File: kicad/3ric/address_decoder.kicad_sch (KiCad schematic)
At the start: 29 parts

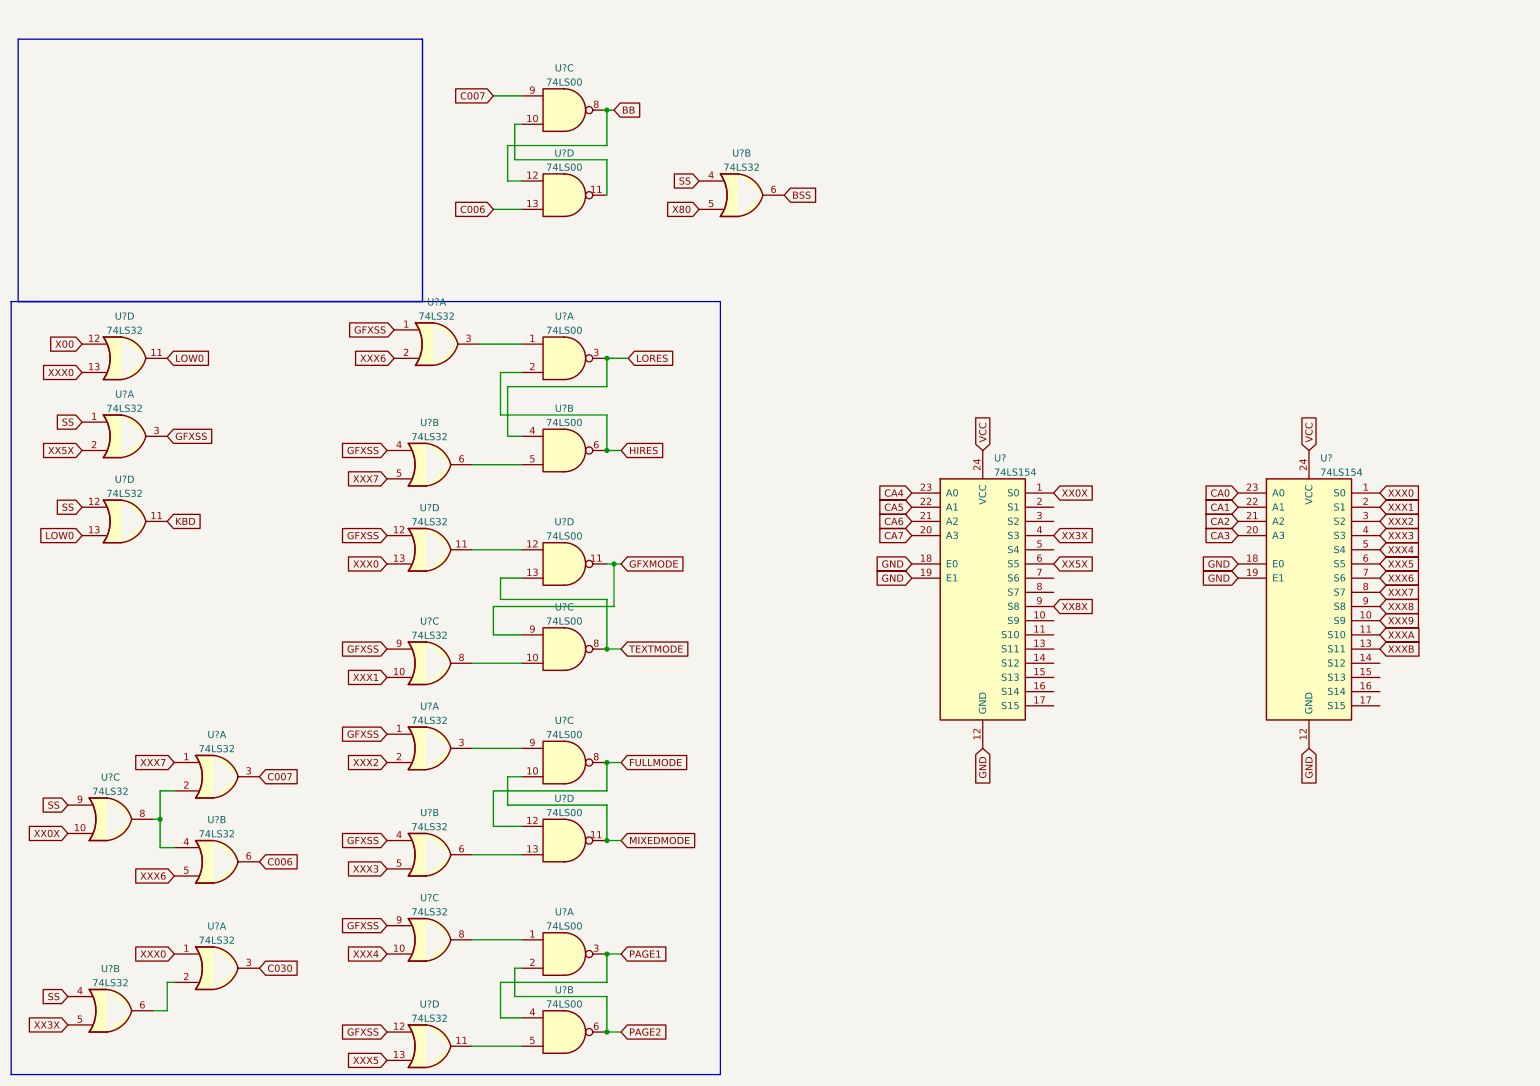
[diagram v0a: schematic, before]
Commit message: push schematic updates
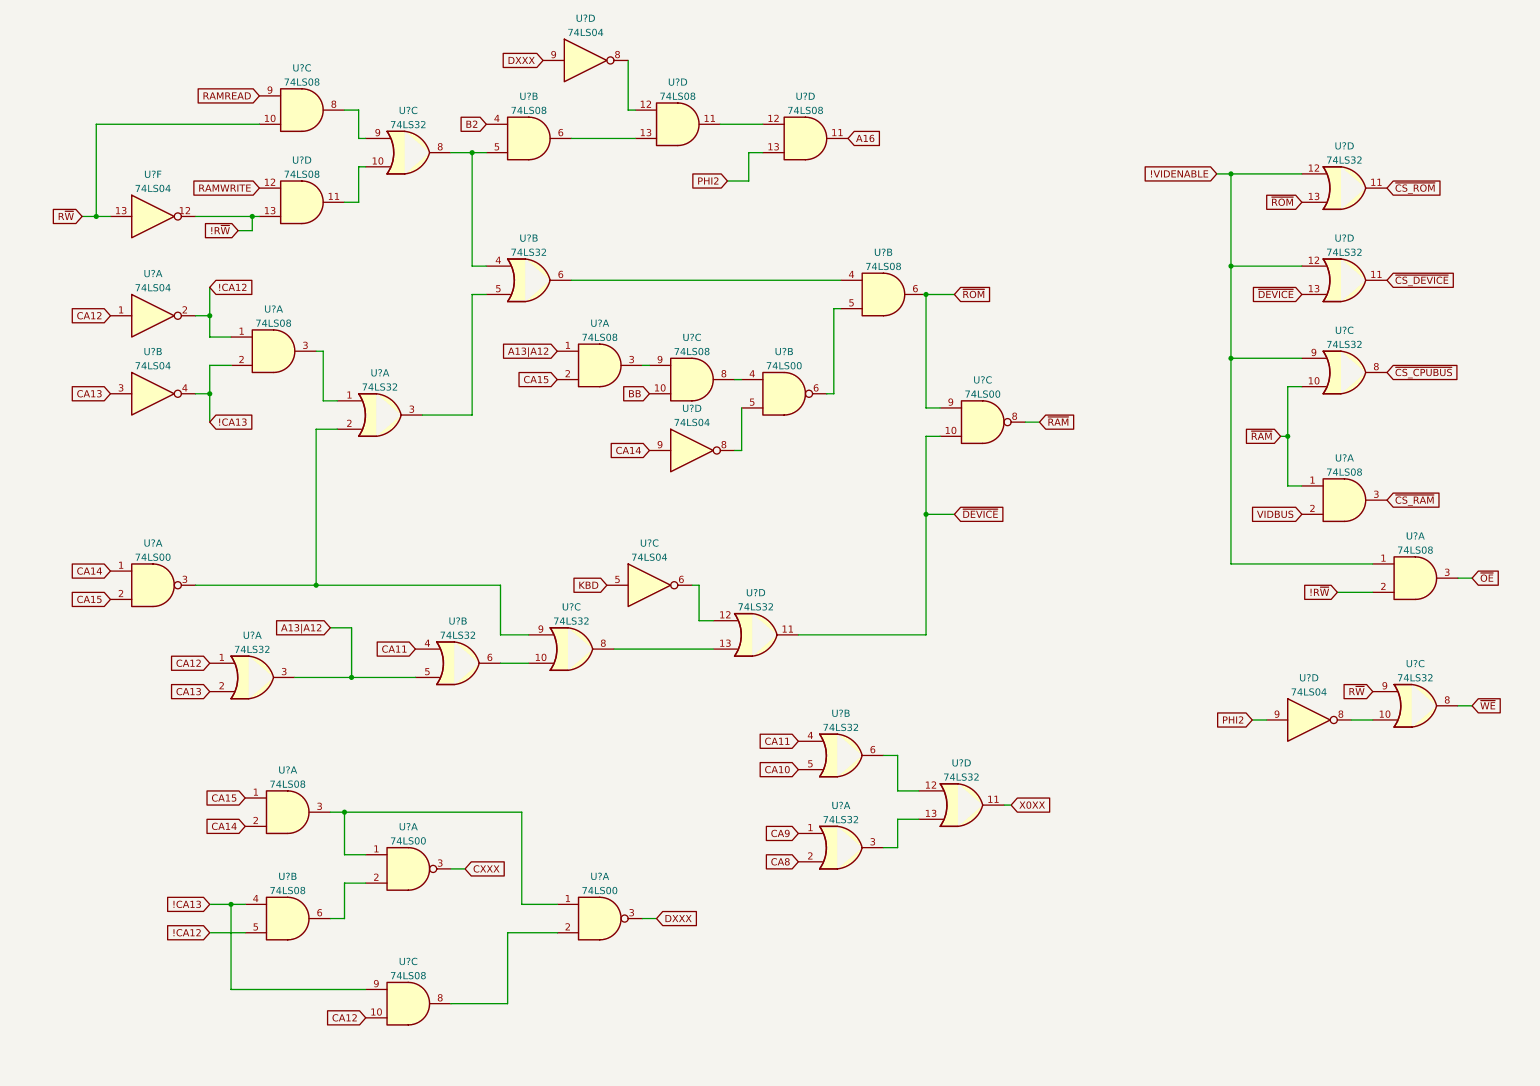
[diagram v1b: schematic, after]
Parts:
- removed U? (x10): 74LS00, symbol 74xx:74LS00
- removed U? (x17): 74LS32, symbol 74xx:74LS32
- removed U? (x2): 74LS154, symbol 74xx:74LS154
- added U? (x7): 74LS04, symbol 74xx:74LS04
- added U? (x14): 74LS32, symbol 74xx:74LS32
- added U? (x14): 74LS08, symbol 74xx:74LS08
- added U? (x5): 74LS00, symbol 74xx:74LS00
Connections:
- net BB: now also U?.10
- net KBD: now also U?.5
- new net: U?.12, U?.6 (x2)
- new net: U?.13, U?.3
- new net: U?.4, U?.8
- new net: U?.3, U?.9
- new net: U?.2, U?.6
- new net: U?.1, U?.1, U?.3
- new net: U?.13, U?.8
- new net: U?.2, U?.8
- new net: U?.11, U?.12
- new net: U?.5, U?.8
- new net: U?.5, U?.6
- new net: U?.8, U?.9
- new net: U?.10, U?.8
- new net: U?.12, U?.8
- new net: U?.10, U?.11
- new net: U?.4, U?.5, U?.8
- new net: U?.13, U?.6
- new net: U?.1, U?.3
- new net: U?.3, U?.5
- new net: U?.4, U?.6
- new net: U?.10, U?.6
- new net: U?.2, U?.3, U?.9
- new net !CA12: U?.1, U?.2, U?.5
- new net !CA13: U?.2, U?.4, U?.4, U?.9
- new net !R~{W}: U?.12, U?.13, U?.2
- new net !VIDENABLE: U?.1, U?.12, U?.12, U?.9
- new net A13|A12: U?.1, U?.3, U?.5
- new net A16: U?.11
- new net B2: U?.4
- new net CA10: U?.5
- new net CA11: U?.4, U?.4
- new net CA12: U?.1, U?.1, U?.10
- new net CA13: U?.2, U?.3
- new net CA14: U?.1, U?.2, U?.9
- new net CA15: U?.1, U?.2, U?.2
- new net CA8: U?.2
- new net CA9: U?.1
- new net CXXX: U?.3
- new net DXXX: U?.3, U?.9
- new net PHI2: U?.13, U?.9
- new net RAMREAD: U?.9
- new net RAMWRITE: U?.12
- new net R~{W}: U?.10, U?.13, U?.9
- new net VIDBUS: U?.2
- new net X0XX: U?.11
- new net ~{CS_CPUBUS}: U?.8
- new net ~{CS_DEVICE}: U?.11
- new net ~{CS_RAM}: U?.3
- new net ~{CS_ROM}: U?.11
- new net ~{DEVICE}: U?.10, U?.11, U?.13
- new net ~{OE}: U?.3
- new net ~{RAM}: U?.1, U?.10, U?.8
- new net ~{ROM}: U?.13, U?.6, U?.9
- new net ~{WE}: U?.8
